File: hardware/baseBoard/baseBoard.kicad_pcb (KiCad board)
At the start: 2 copper layers, 120 x 90 mm, 30 parts, among them J1 Screw_Terminal_01x06, Q1 BC817, U1 Finder66.22, U2 MCP601-xOT, U3 CS1XXX, U4 AP65111AWU

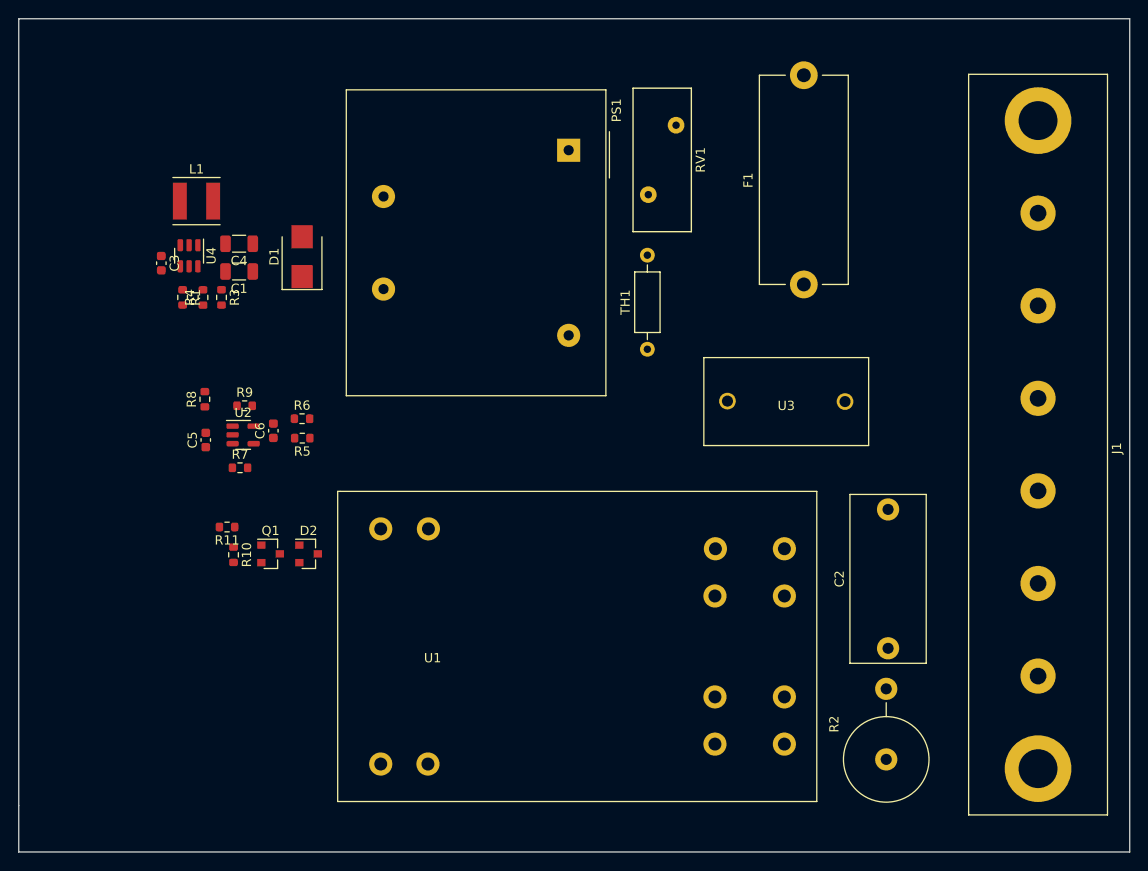
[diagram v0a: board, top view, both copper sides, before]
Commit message: sch / pcb update
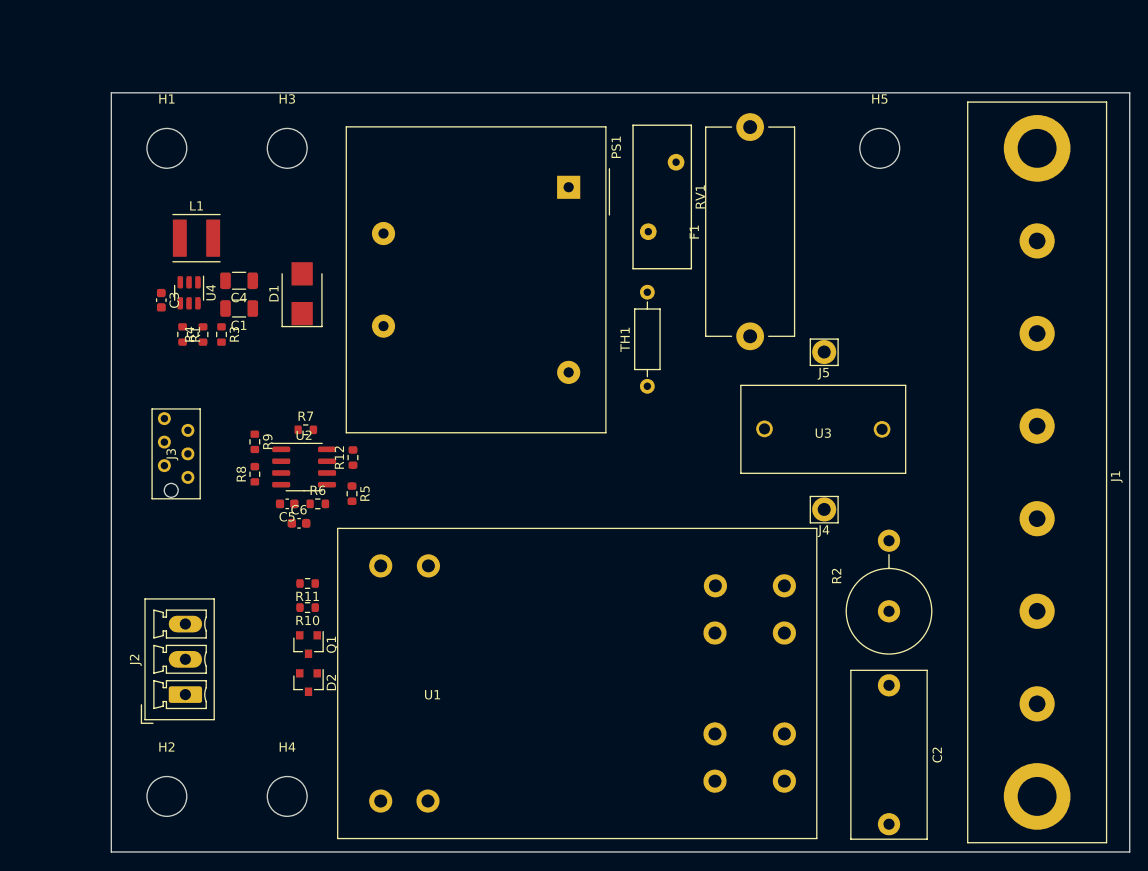
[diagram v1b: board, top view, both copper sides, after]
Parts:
- added H1: MountingHole, MountingHole:MountingHole_4.3mm_M4, F.Cu at (76.0, 49.0)
- added H2: MountingHole, MountingHole:MountingHole_4.3mm_M4, F.Cu at (76.0, 119.0)
- added H3: MountingHole, MountingHole:MountingHole_4.3mm_M4, F.Cu at (89.0, 49.0)
- added H4: MountingHole, MountingHole:MountingHole_4.3mm_M4, F.Cu at (89.0, 119.0)
- added H5: MountingHole, MountingHole:MountingHole_4.3mm_M4, F.Cu at (153.0, 49.0)
- added J2: Conn_01x03, Connector_Phoenix_MC:PhoenixContact_MCV_1,5_3-G-3.81_1x03_P3.81mm_Vertical, F.Cu at (78.0, 108.0)
- added J3: Conn_01x06, baseBoard:2178710-6, F.Cu at (77.0, 82.0)
- added J4: Conn_01x01, Connector_Pin:Pin_D1.4mm_L8.5mm_W2.8mm_FlatFork, F.Cu at (147.0, 88.0)
- added J5: Conn_01x01, Connector_Pin:Pin_D1.4mm_L8.5mm_W2.8mm_FlatFork, F.Cu at (147.0, 71.0)
- added R12: tbd, Resistor_SMD:R_0603_1608Metric, F.Cu at (96.1, 82.4)
- R6: value tbd -> 75k
- U2: value MCP601-xOT -> MCP6L02x-xSN; footprint Package_TO_SOT_SMD:SOT-23-5 -> Package_SO:SOIC-8_3.9x4.9mm_P1.27mm
- moved R2 16.0 mm to (154.0, 99.0)
- moved D2 13.9 mm to (91.3, 106.7), turned to 270 degrees
- moved C5 11.2 mm to (89.0, 87.4), turned to 180 degrees
- moved R11 10.6 mm to (91.2, 96.0)
- moved Q1 10.6 mm to (91.3, 102.6), turned to 270 degrees
- moved C6 10.4 mm to (90.3, 89.5), turned to 0 degrees
- moved R10 9.82 mm to (91.2, 98.6), turned to 180 degrees
- moved R8 9.73 mm to (85.5, 84.2)
- moved R6 9.36 mm to (92.3, 87.4)
- moved R7 8.20 mm to (91.0, 79.4)
- moved F1 8.06 mm to (139.0, 69.3)
- moved R5 8.06 mm to (96.0, 86.3), turned to 270 degrees
- moved U2 7.45 mm to (90.8, 83.4)
- moved U3 5.00 mm to (146.9, 79.3)
- moved R9 4.05 mm to (85.5, 80.7), turned to 270 degrees
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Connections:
- R11 pad 2: (no net) -> /REL_SW
- U1 pad 11: /N -> Net-(J4-Pad1)
- U1 pad 14: /N_MOTOR -> /L_MOTOR
- U1 pad 21: /L -> /N
- U1 pad 24: /L_MOTOR -> /N_MOTOR
- U2 pad 2: GND -> Net-(R8-Pad2)
- U2 pad 4: Net-(R8-Pad2) -> GND
- U2 pad 5: +5V -> Net-(R5-Pad1)
- U3 pad 3: Net-(R5-Pad1) -> Net-(R12-Pad1)
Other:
- board size 120 x 90 mm -> 110 x 82 mm
